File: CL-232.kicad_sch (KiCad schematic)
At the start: 42 parts, among them J1 Conn_01x06, J2 Screw_Terminal_01x10, J3 Barrel_Jack_Switch, J4 DE9_Socket, Q1 2N3904, Q2 2N3904, Q3 2N3904, Q4 2N3906, Q5 2N3904, U1 6N135, U2 4N35, U3 LM7805_TO220, U4 MAX3232

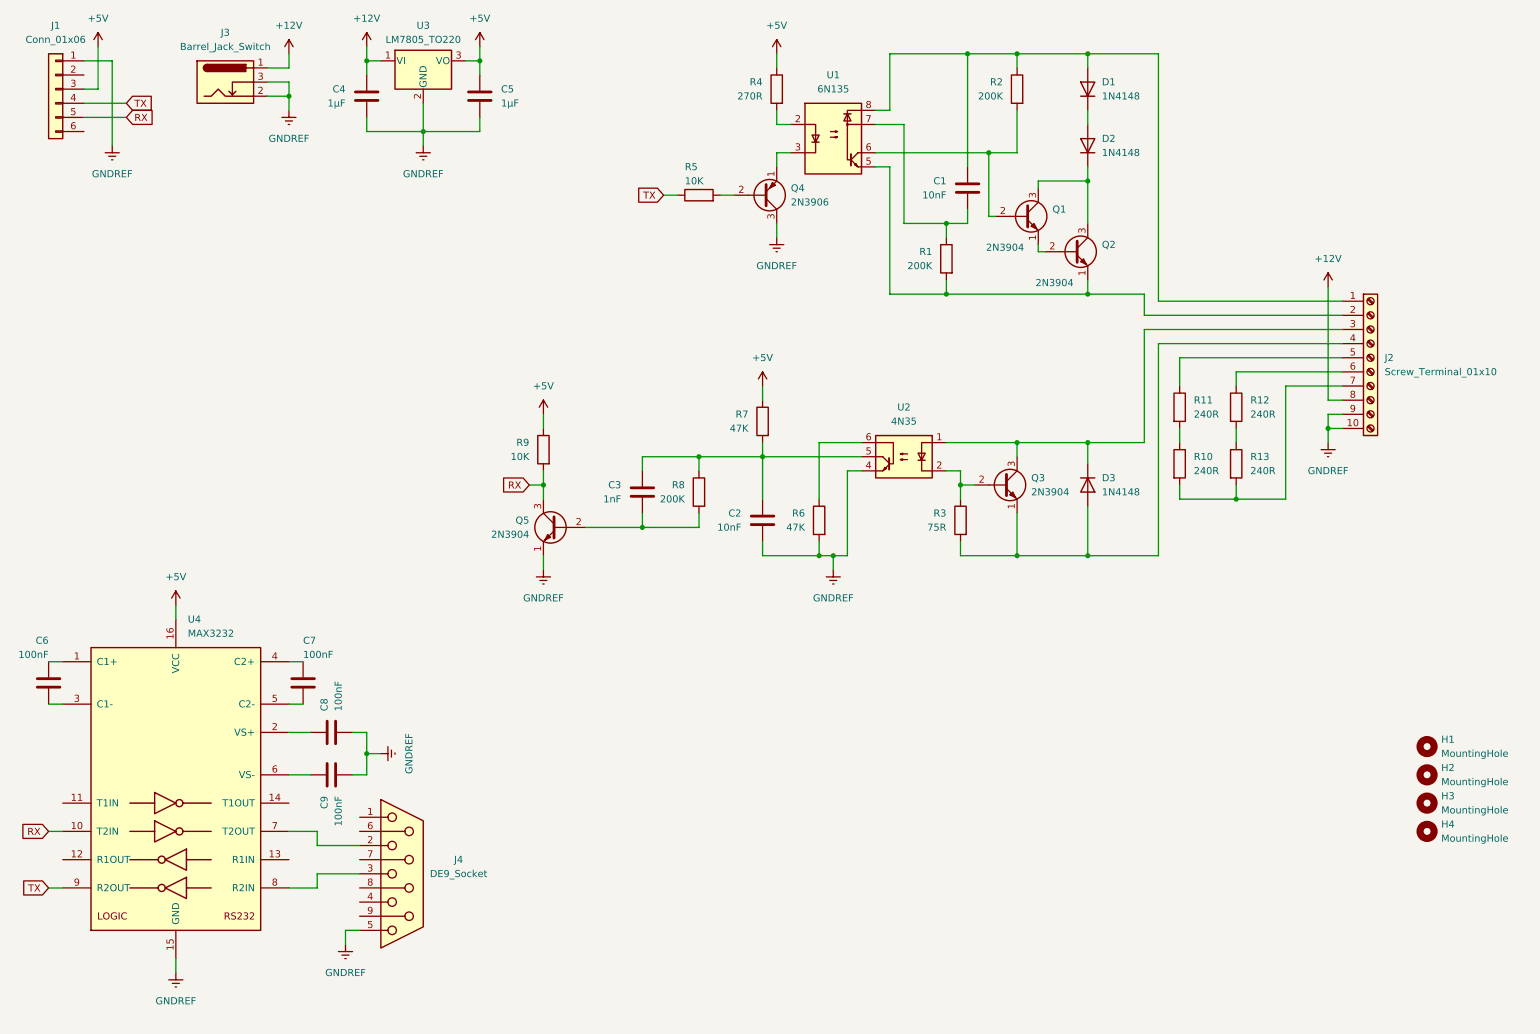
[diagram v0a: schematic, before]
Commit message: 2025-12-30 21:43
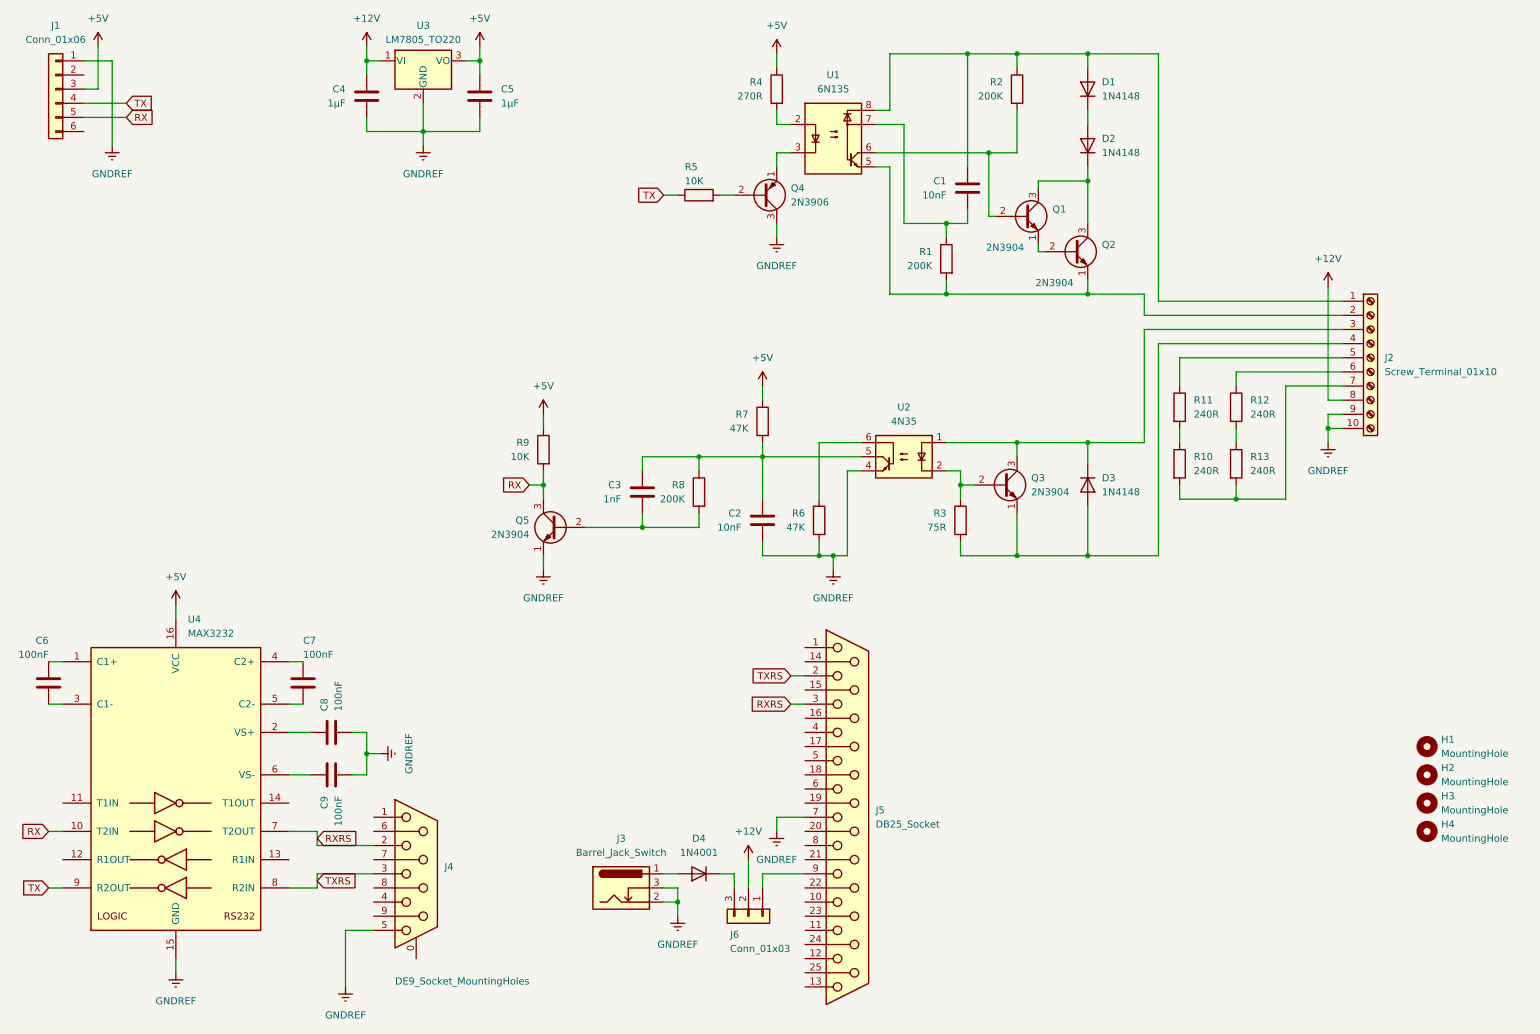
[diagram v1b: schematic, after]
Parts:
- removed J4: DE9_Socket, Connector_Dsub:DSUB-9_Socket_Horizontal_P2.77x2.84mm_EdgePinOffset4.94mm_Housed_MountingHolesOffset4.94mm, symbol Connector:DE9_Socket
- added D4: 1N4001, Diode_THT:D_DO-41_SOD81_P2.54mm_Vertical_AnodeUp, symbol Diode:1N4001
- added J4: DE9_Socket_MountingHoles, Connector_Dsub:DSUB-9_Socket_Horizontal_P2.77x2.84mm_EdgePinOffset4.94mm_Housed_MountingHolesOffset4.94mm, symbol Connector:DE9_Socket_MountingHoles
- added J5: DB25_Socket, Connector_Dsub:DSUB-25_Socket_EdgeMount_P2.77mm, symbol Connector:DB25_Socket
- added J6: Conn_01x03, Connector_PinHeader_2.54mm:PinHeader_1x03_P2.54mm_Vertical, symbol Connector_Generic:Conn_01x03
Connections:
- net +12V: now also J6.2 (Pin_2); no longer J3.1
- net GNDREF: now also J4.5, J5.7
- net RXRS: now reaches U4.7 (T2OUT)
- net RXRS: now also J4.2, J5.3
- net TXRS: now reaches U4.8 (R2IN)
- net TXRS: now also J4.3, J5.2
- new net: D4.2 (A), J3.1
- new net: J5.9, J6.1 (Pin_1)
- new net: D4.1 (K), J6.3 (Pin_3)
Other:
- moved on the sheet: J3
